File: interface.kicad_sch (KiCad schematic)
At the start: 6 parts, among them J1 SJ-3524-SMT-TR, U1 2.42OLED

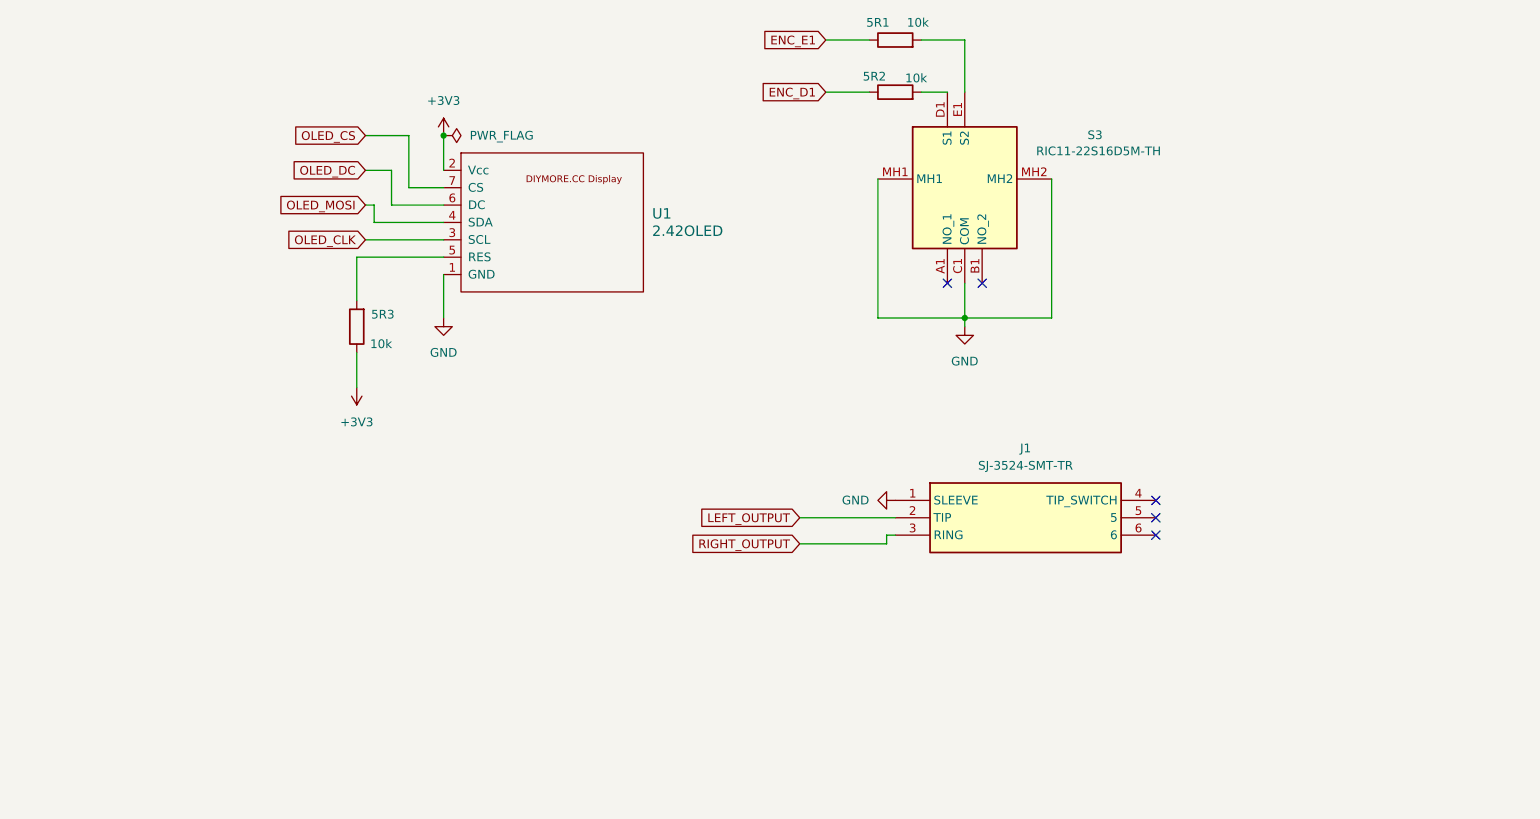
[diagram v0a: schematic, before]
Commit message: finalized schema
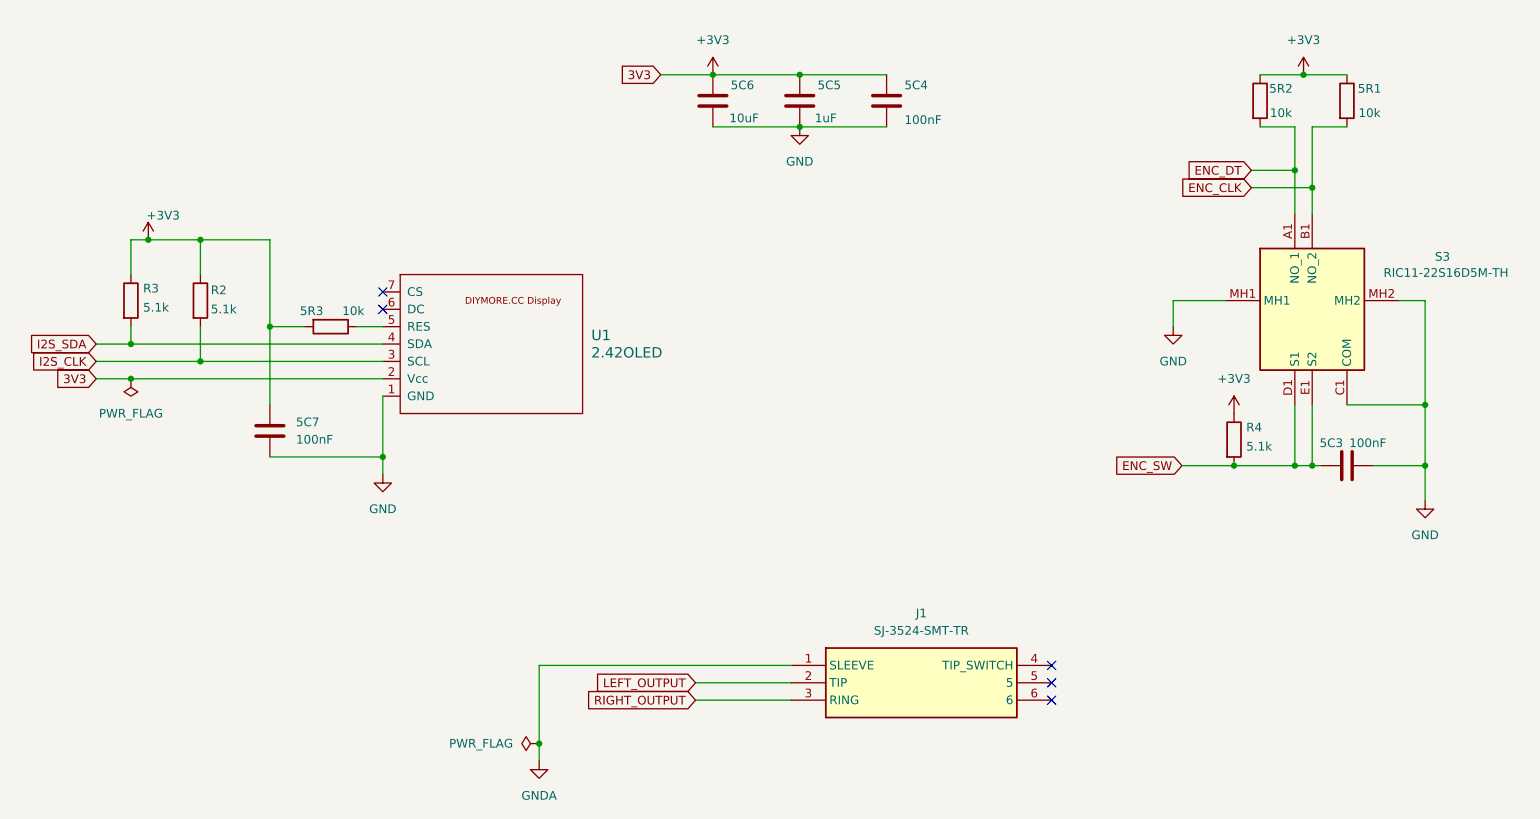
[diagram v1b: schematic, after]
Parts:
- added 5C3, 5C4, 5C7: 100nF, Capacitor_SMD:C_0402_1005Metric, symbol Device:C
- added 5C5: 1uF, Capacitor_SMD:C_0402_1005Metric, symbol Device:C
- added 5C6: 10uF, Capacitor_SMD:C_0402_1005Metric, symbol Device:C
- added R2, R3, R4: 5.1k, Resistor_SMD:R_0402_1005Metric, symbol Device:R
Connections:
- net ENC_D1 is gone; now on net +3V3: 5R2.1
- net ENC_E1 is gone; now on net +3V3: 5R1.1
- net +3V3: now also 5R3.2, 5C4.2, 5C5.2, 5C6.2, 5C7.1, R2.1, R3.1, R4.1; no longer 5R3.1
- net GND: now also 5C3.2, 5C4.1, 5C5.1, 5C6.1, 5C7.2; no longer J1.1 (SLEEVE)
- net ENC_DT: now reaches 5R2.2
- net ENC_DT: now also S3.A1 (NO_1); no longer S3.D1 (S1)
- net ENC_CLK: now reaches 5R1.2
- net ENC_CLK: now also S3.B1 (NO_2); no longer S3.E1 (S2)
- net at U1.5 (RES): now also 5R3.1; no longer 5R3.2
- net OLED_CLK renamed I2S_CLK
- net I2S_CLK: now also R2.2
- net OLED_CS: no longer names the net of U1.7 (CS)
- net OLED_DC: no longer names the net of U1.6 (DC)
- net OLED_MOSI renamed I2S_SDA
- net I2S_SDA: now also R3.2
- new net ENC_SW: 5C3.1, R4.2, S3.D1 (S1), S3.E1 (S2)
- new net GNDA: J1.1 (SLEEVE)
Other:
- moved on the sheet: 5R1, 5R2, 5R3, J1, S3, U1
